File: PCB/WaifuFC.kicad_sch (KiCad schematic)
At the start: 58 parts, among them J1 SBUS, J2 USB_C_Receptacle_USB2.0, J3 PPM, J4 OUT, J5 Conn_01x02, J6 Conn_01x02, J7 Conn_01x04, Q1 1P, SW1 SW_Push, U1 STM32F103C8Tx, U2 MPU-6050, U3 MP1584, U4 AZ1117-3.3, Y1 8MHz

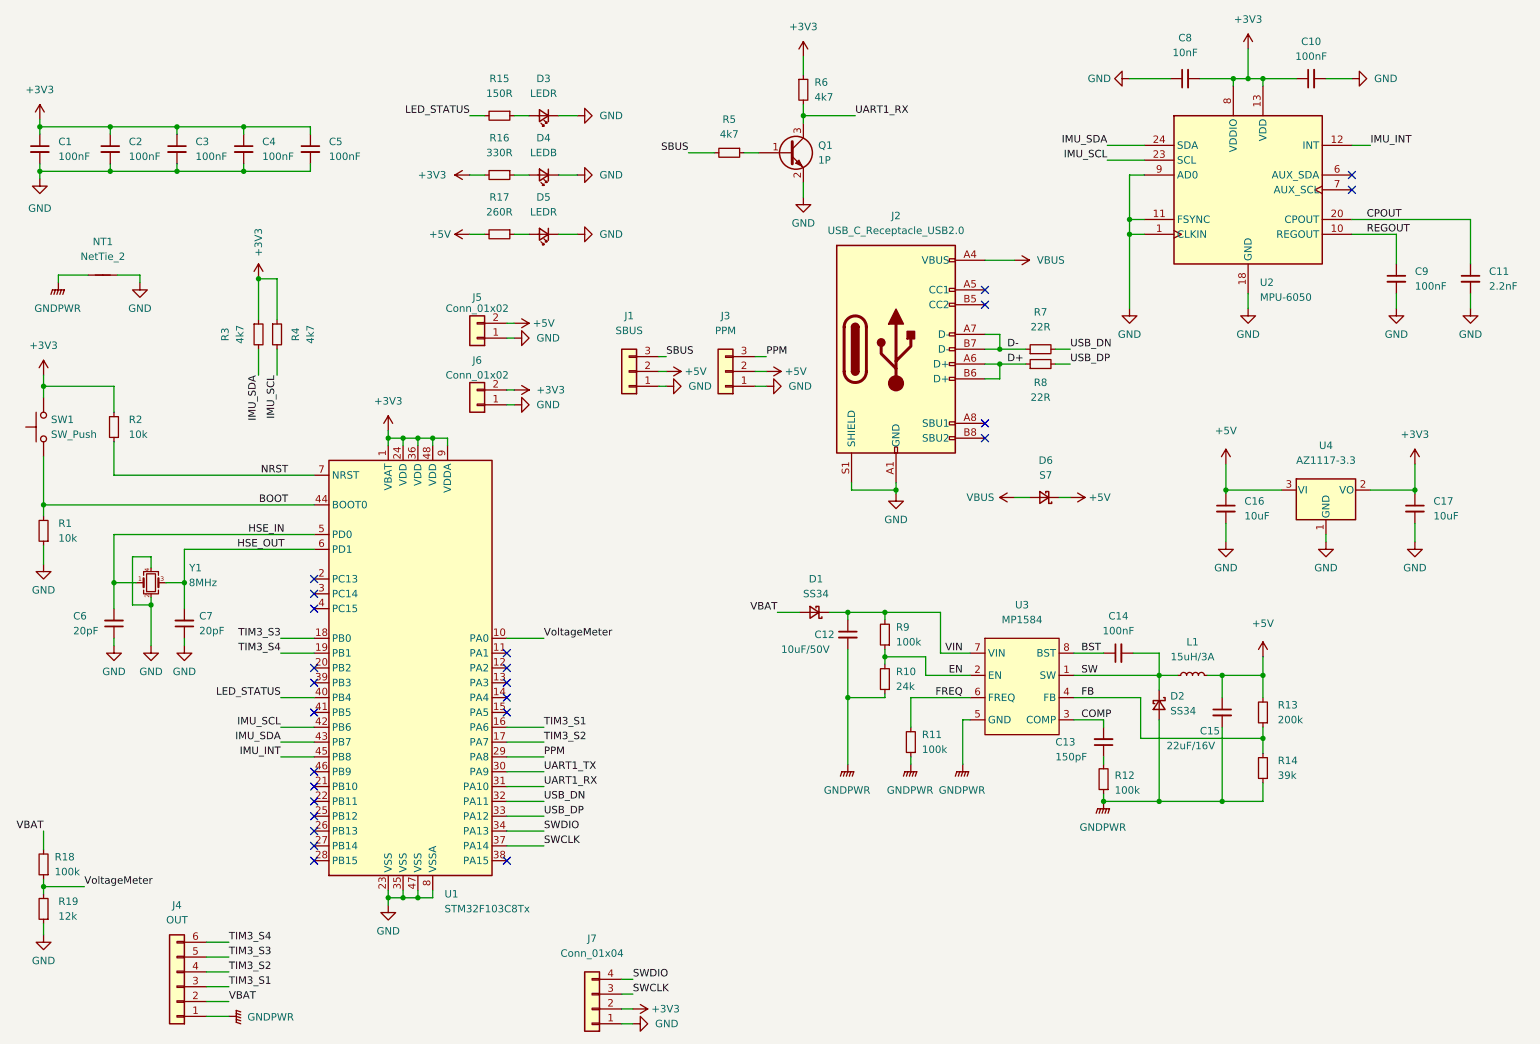
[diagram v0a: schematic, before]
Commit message: v3
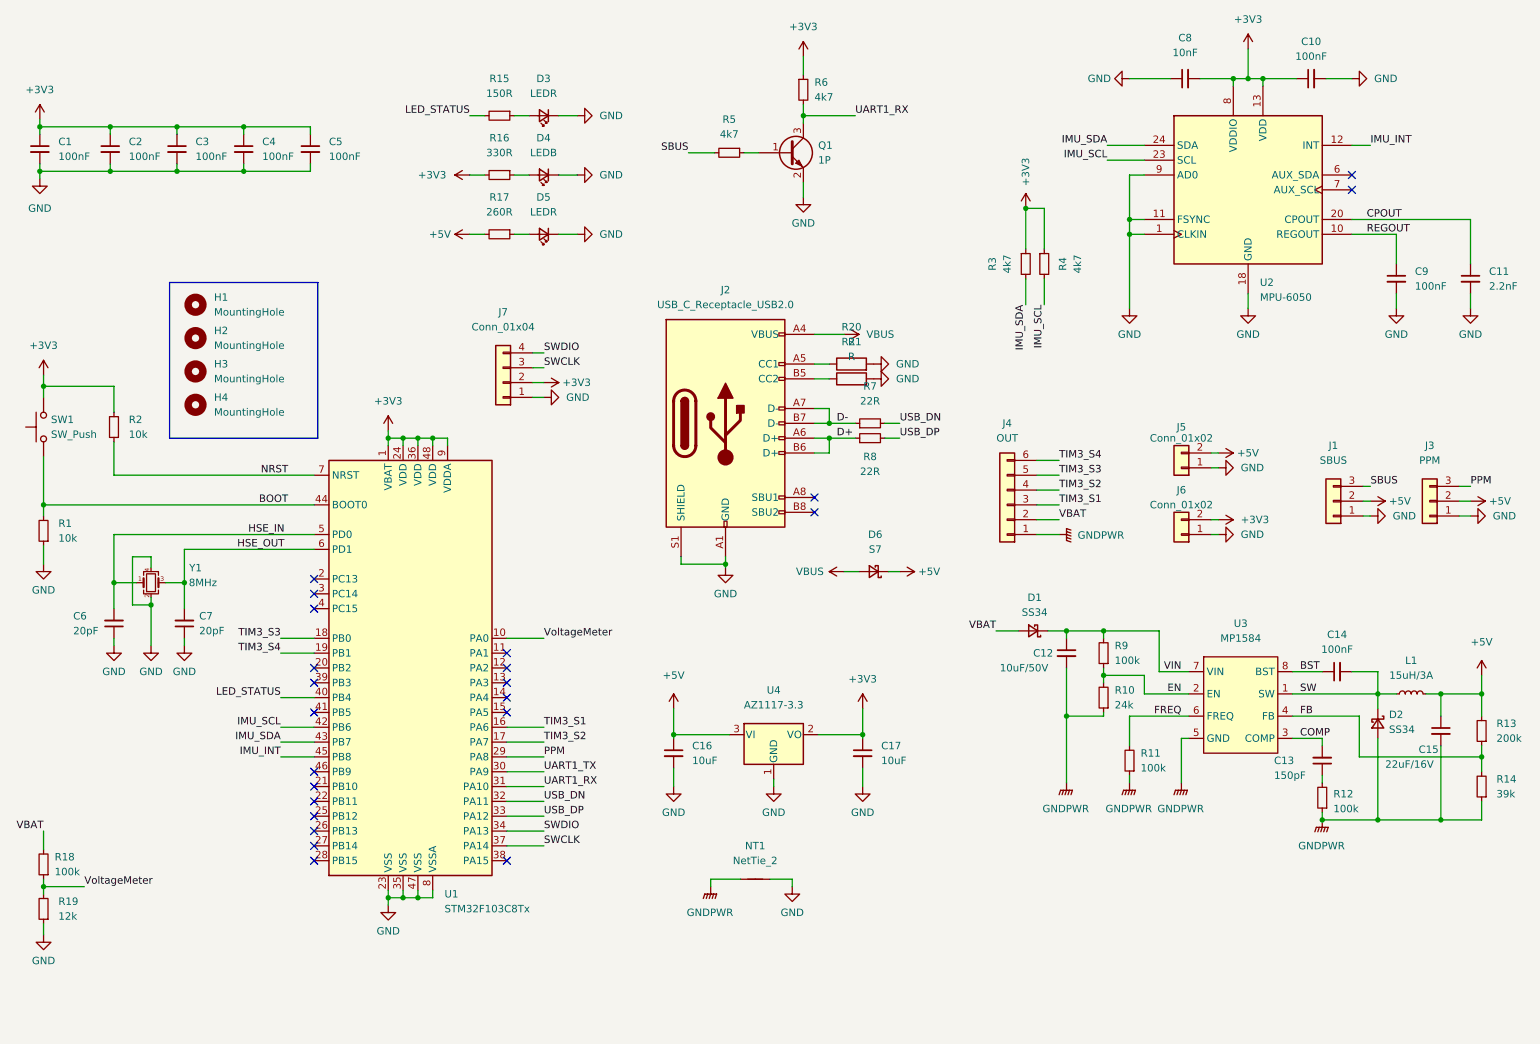
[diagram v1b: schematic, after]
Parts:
- added H1, H2, H3, H4: MountingHole, MountingHole:MountingHole_3mm_Pad, symbol Mechanical:MountingHole
- added R20, R21: R, Resistor_SMD:R_0402_1005Metric, symbol Device:R
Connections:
- net GND: now also R20.2, R21.2
- net at J2.A5 (CC1): now also R20.1
- net at J2.B5 (CC2): now also R21.1
- no-connect marks 25 -> 23
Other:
- title: (none) -> Waifu FC 2.0
- moved on the sheet: C12, C13, C14, C15, C16, C17, D1, D2, D6, J1, J2, J3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

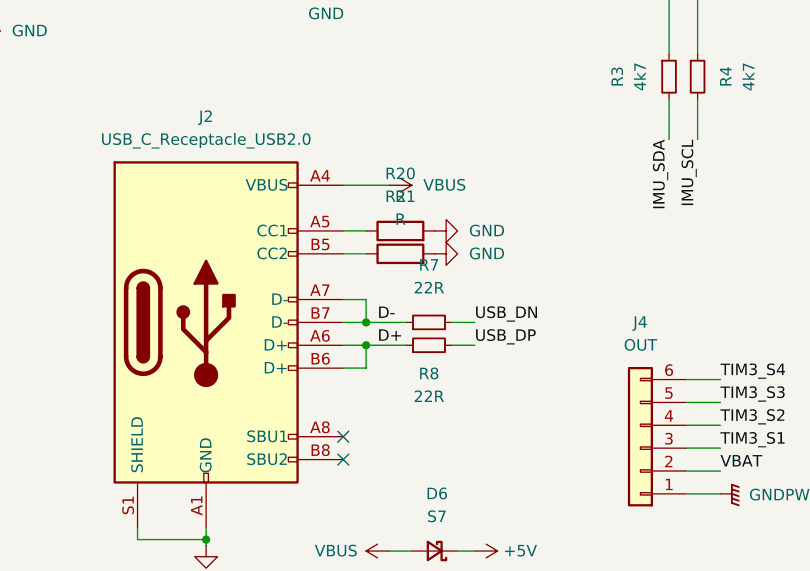
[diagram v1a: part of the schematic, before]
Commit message: elowina
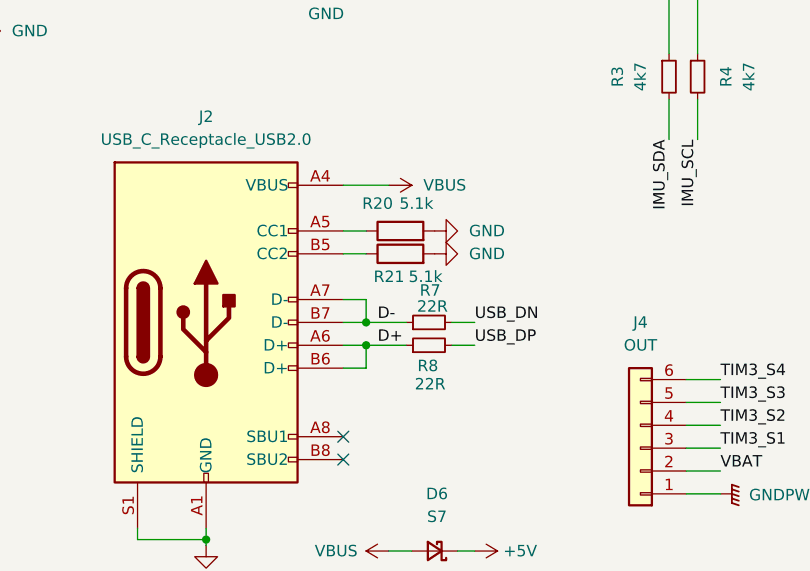
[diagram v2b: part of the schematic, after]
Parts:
- R20, R21: value R -> 5.1k
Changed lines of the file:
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@@
 		(on_board yes)
 		(dnp no)
-		(fields_autoplaced yes)
 		(property "Reference" "R20"
-			(at 163.83 71.12 90)
+			(at 161.29 74.422 90)
 			(effects
 				(font
@@
 			)
 		)
-		(property "Value" "R"
-			(at 163.83 73.66 90)
+		(property "Value" "5.1k"
+			(at 165.608 74.422 90)
 			(effects
 				(font
@@
 		(on_board yes)
 		(dnp no)
-		(fields_autoplaced yes)
 		(property "Reference" "R21"
-			(at 163.83 73.66 90)
+			(at 162.56 82.55 90)
 			(effects
 				(font
@@
 			)
 		)
-		(property "Value" "R"
-			(at 163.83 76.2 90)
+		(property "Value" "5.1k"
+			(at 166.624 82.55 90)
 			(effects
 				(font
@@
 		(dnp no)
 		(property "Reference" "R8"
-			(at 167.005 93.345 90)
+			(at 166.878 92.456 90)
 			(effects
 				(font
@@
 		)
 		(property "Value" "22R"
-			(at 167.005 95.885 90)
+			(at 167.132 94.488 90)
 			(effects
 				(font
@@
 		(on_board yes)
 		(dnp no)
-		(fields_autoplaced yes)
 		(property "Reference" "R7"
-			(at 167.005 81.28 90)
+			(at 167.132 84.074 90)
 			(effects
 				(font
@@
 		)
 		(property "Value" "22R"
-			(at 167.005 83.82 90)
+			(at 167.386 85.852 90)
 			(effects
 				(font
